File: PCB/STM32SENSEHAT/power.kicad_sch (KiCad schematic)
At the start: 18 parts, among them IC1 DW01A, Q1 NMOS, Q2 NMOS, U1 MCP1700x-330xxTT, U2 TP4056

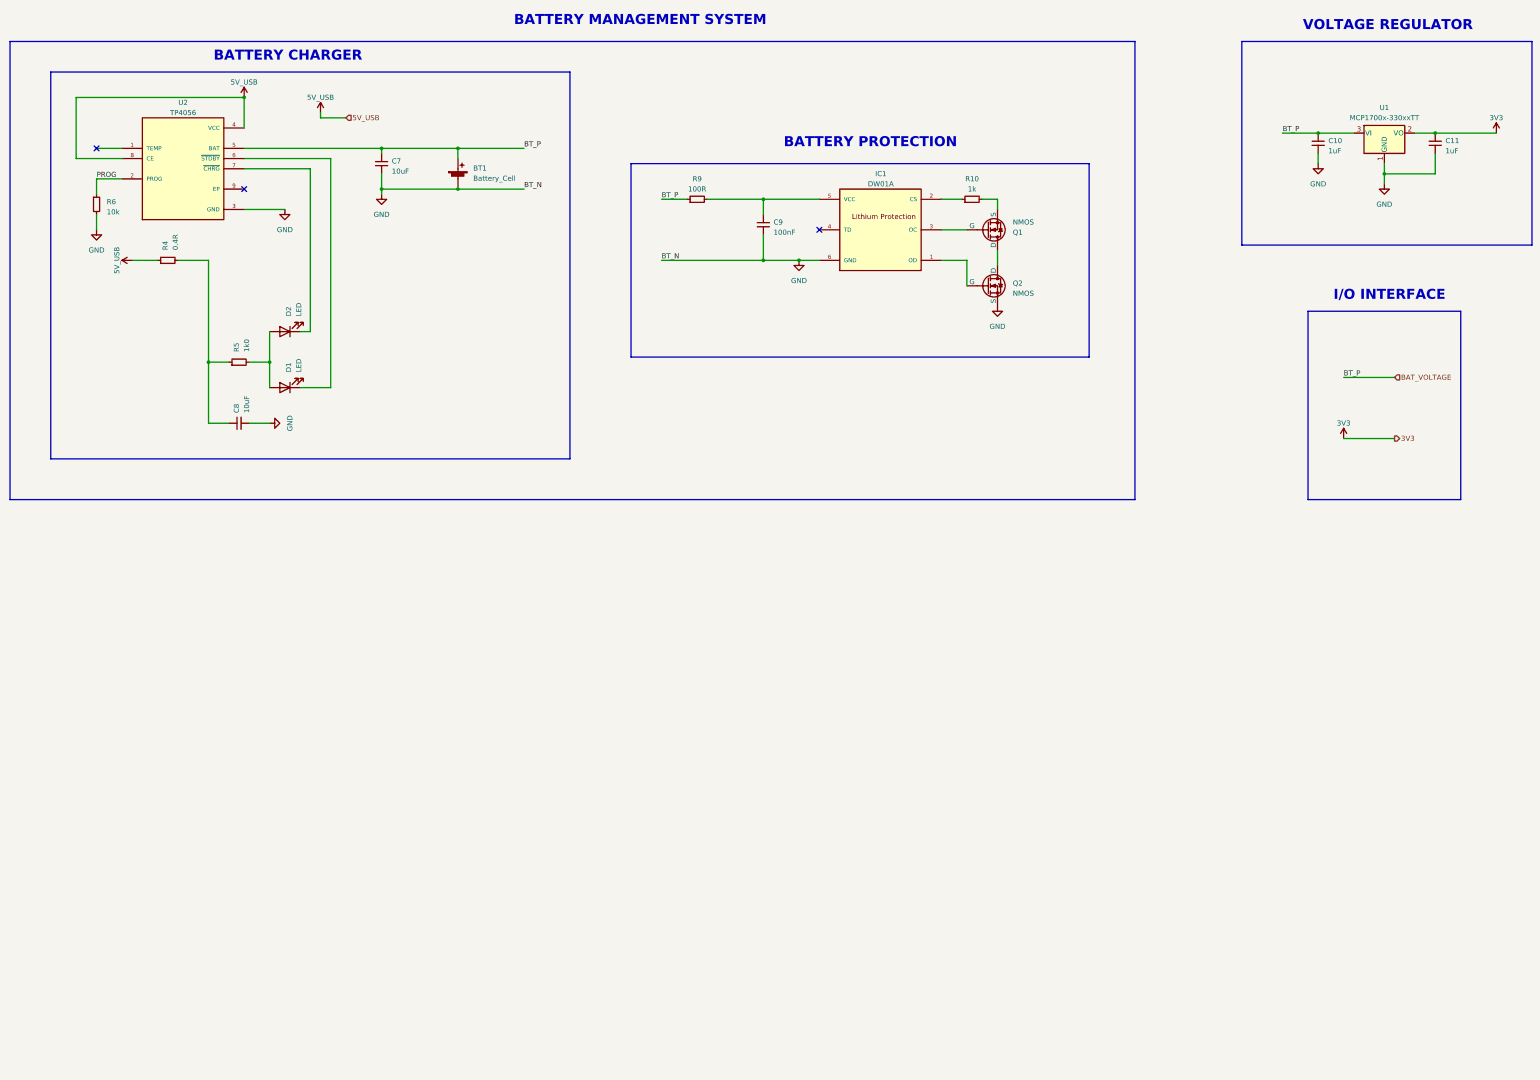
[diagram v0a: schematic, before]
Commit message: Protectuion features added to all schematica
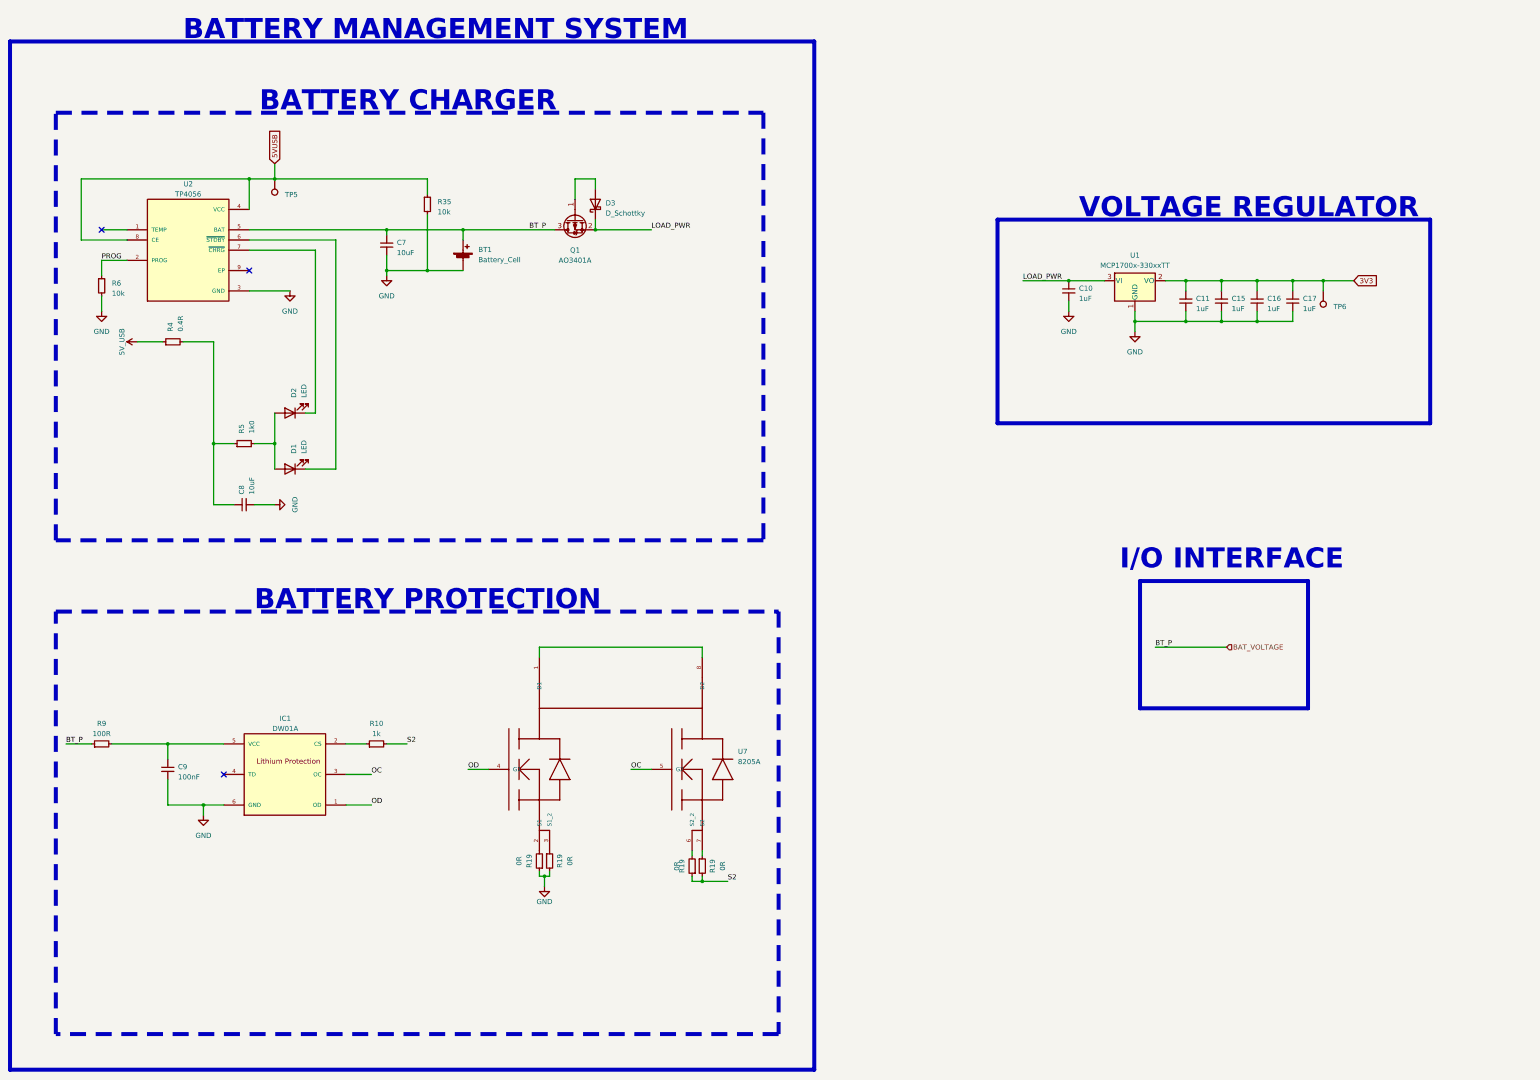
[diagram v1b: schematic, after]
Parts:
- removed Q1, Q2: NMOS, symbol Simulation_SPICE:NMOS
- added C15, C16, C17: 1uF, symbol Device:C_Small
- added D3: D_Schottky, symbol Device:D_Schottky
- added Q1: AO3401A, Package_TO_SOT_SMD:SOT-23, symbol Transistor_FET:AO3401A
- added R19 (x4): 0R, symbol Device:R_Small
- added R35: 10k, symbol Device:R_Small
- added TP5, TP6: TestPoint, symbol Connector:TestPoint
- added U7: 8205A, TSSOP8, symbol 8205A:8205A
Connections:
- net BAT_VOLTAGE: now also Q1.3 (D); no longer C10.1, U1.3 (VI)
- net GND: now also C15.2, C16.2, C17.2, R19.1, R19.2, R35.2
- net VCC: no longer C11.1, U1.2 (VO), U2.4 (VCC), U2.8 (CE)
- net OD: now reaches IC1.1 (OD)
- net OD: now also U7.4 (G1)
- net S2: now reaches R10.2
- net S2: now also R19.1, R19.2
- net OC: now reaches IC1.3 (OC)
- net OC: now also U7.5 (G2)
- new net: U7.1 (D1), U7.8 (D2)
- new net: R19.2, U7.2 (S1)
- new net: R19.1, U7.3 (S1_2)
- new net: R19.2, U7.6 (S2_2)
- new net: R19.1, U7.7 (S2)
- new net: D3.2 (A), Q1.1 (G)
- new net 3V3: C11.1, C15.1, C16.1, C17.1, TP6.1, U1.2 (VO)
- new net 5VUSB: R35.1, TP5.1, U2.4 (VCC), U2.8 (CE)
- new net LOAD_PWR: C10.1, D3.1 (K), Q1.2 (S), U1.3 (VI)
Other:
- moved on the sheet: BT1, C10, C11, C7, C8, C9, D1, D2, IC1, R10, R4, R5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
